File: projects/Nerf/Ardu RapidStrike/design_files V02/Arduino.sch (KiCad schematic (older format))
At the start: 73 parts, among them J1 BATT_OUT, J10 PWM_IN, J11 PWM_OUT, J12 CLIP, J14 NPTH, J15 BATT, J16 NPTH, J17 PSH_IN, J18 PSH_OUT, J19 TRIG, J2 BATT_IN, J20 PUSH, J21 BUTTON, J22 TRIG_OUT, J23 TRIG_IN, J24 TO_IR, J25 PHOTO, J26 IR_LED, J27 BUTTON, J3 PUSHER, J4 JAM, J5 I2C, J6 REV, J7 FTDI, J8 PHOTO, J9 FLYWHEELS, Q1 IRLB8721, Q2 Photo_NPN, SW1 SW_Rotary8, SW2 SW_Push, U1 MCP1702, U2 L293D, U3 HALL SENSOR, U4 HALL SENSOR, U5 ATMEGA328P-PU, U6 HALL SENSOR, U7 74LS14, Y1 16Mhz

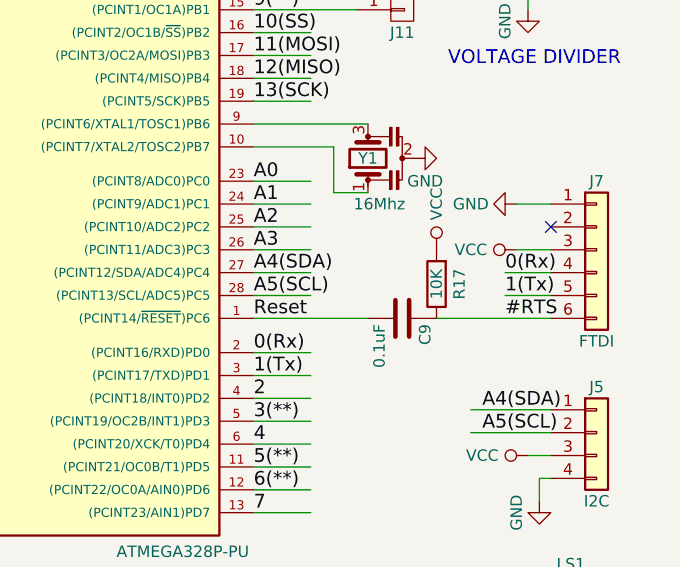
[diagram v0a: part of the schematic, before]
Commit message: Updates
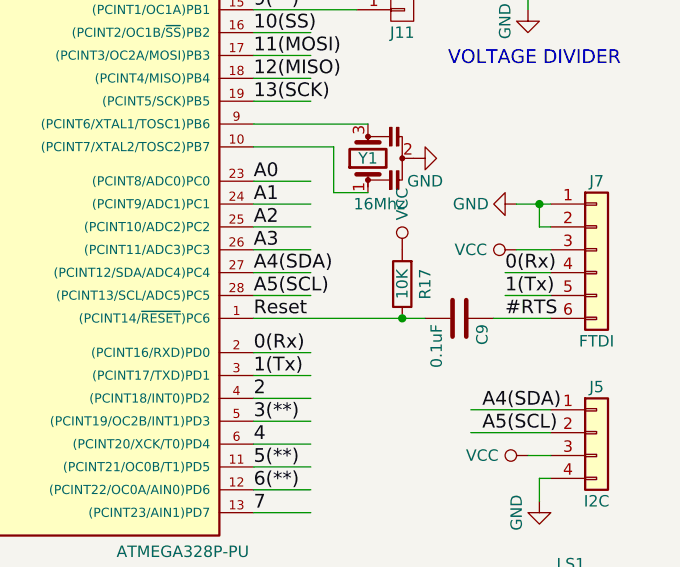
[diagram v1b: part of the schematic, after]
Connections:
- wire segments 211 -> 213
- no-connect marks 4 -> 3
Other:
- moved on the sheet: C9, R17
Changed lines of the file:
@@
 	1    0    0    -1
 $EndComp
-NoConn ~ 10050 3500
 Text Label 9850 3800 0    60   ~ 0
 1(Tx)
@@
 L C C9
 U 1 1 5CF78490
-P 9400 3900
-F 0 "C9" H 9425 4000 50  0000 L CNN
-F 1 "0.1uF" H 9425 3800 50  0000 L CNN
-F 2 "footprints:C_Disc_D3.4mm_W2.1mm_P2.50mm" H 9438 3750 50  0001 C CNN
-F 3 "" H 9400 3900 50  0001 C CNN
-	1    9400 3900
+P 9650 3900
+F 0 "C9" H 9675 4000 50  0000 L CNN
+F 1 "0.1uF" H 9675 3800 50  0000 L CNN
+F 2 "footprints:C_Disc_D3.4mm_W2.1mm_P2.50mm" H 9688 3750 50  0001 C CNN
+F 3 "" H 9650 3900 50  0001 C CNN
+	1    9650 3900
 	0    1    1    0
 $EndComp
@@
 L R R17
 U 1 1 5CF785A0
-P 9550 3750
-F 0 "R17" V 9450 3750 50  0000 C CNN
-F 1 "10K" V 9550 3750 50  0000 C CNN
-F 2 "footprints:R__P5.08mm" V 9480 3750 50  0001 C CNN
-F 3 "" H 9550 3750 50  0001 C CNN
-	1    9550 3750
+P 9400 3750
+F 0 "R17" V 9300 3750 50  0000 C CNN
+F 1 "10K" V 9400 3750 50  0000 C CNN
+F 2 "footprints:R__P5.08mm" V 9330 3750 50  0001 C CNN
+F 3 "" H 9400 3750 50  0001 C CNN
+	1    9400 3750
 	-1   0    0    1
 $EndComp
@@
 L VCC #PWR032
 U 1 1 5CF7868B
-P 9550 3600
-F 0 "#PWR032" H 9550 3450 50  0001 C CNN
-F 1 "VCC" V 9550 3800 50  0000 C CNN
-F 2 "" H 9550 3600 50  0001 C CNN
-F 3 "" H 9550 3600 50  0001 C CNN
-	1    9550 3600
+P 9400 3600
+F 0 "#PWR032" H 9400 3450 50  0001 C CNN
+F 1 "VCC" V 9400 3800 50  0000 C CNN
+F 2 "" H 9400 3600 50  0001 C CNN
+F 3 "" H 9400 3600 50  0001 C CNN
+	1    9400 3600
 	1    0    0    -1
 $EndComp
@@
 Wire Wire Line
 	5250 4600 5400 4600
-Wire Wire Line
-	9550 3900 10050 3900
 Connection ~ 5250 1750
 Wire Wire Line
@@
 	1900 1050 1900 1150
 Wire Wire Line
-	8750 3900 9250 3900
+	8750 3900 9500 3900
 Wire Wire Line
 	10000 900  10150 900
@@
 Text Notes 5650 1150 0    60   ~ 0
 1.25V\n256
+Connection ~ 9400 3900
+Wire Wire Line
+	9800 3900 10050 3900
+Wire Wire Line
+	10050 3500 10000 3500
+Wire Wire Line
+	10000 3500 10000 3400
+Connection ~ 10000 3400
 $EndSCHEMATC
